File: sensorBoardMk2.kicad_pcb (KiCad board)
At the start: 2 copper layers, 42.3 x 63 mm, 45 parts, among them J1 S4B-PH-K-S__LF__SN_, J2 S4B-PH-K-S__LF__SN_, P1 TP, P2 TP, P3 TP, P4 TP, P5 TP, U1 SHT45, U2 BME280, U3 SGP40-D-R4

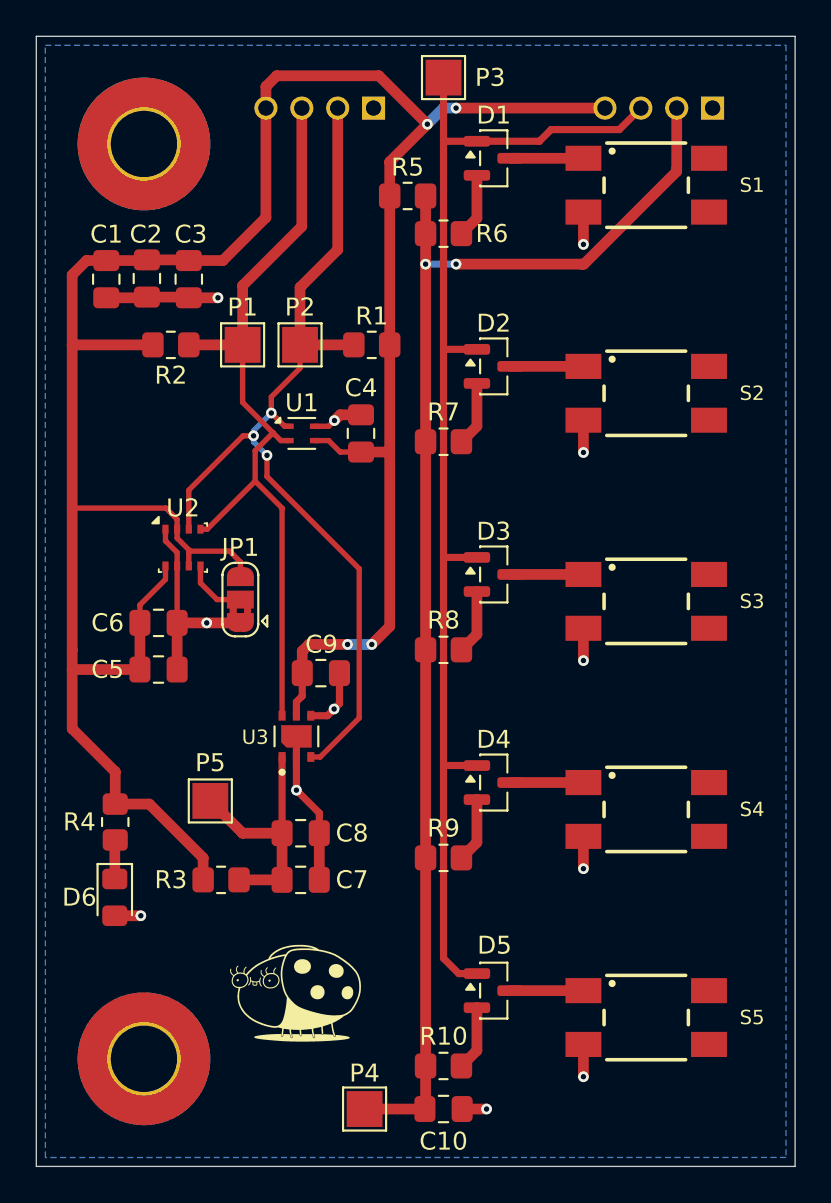
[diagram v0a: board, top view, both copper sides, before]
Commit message: Did some improvements based on feedback from lil brother
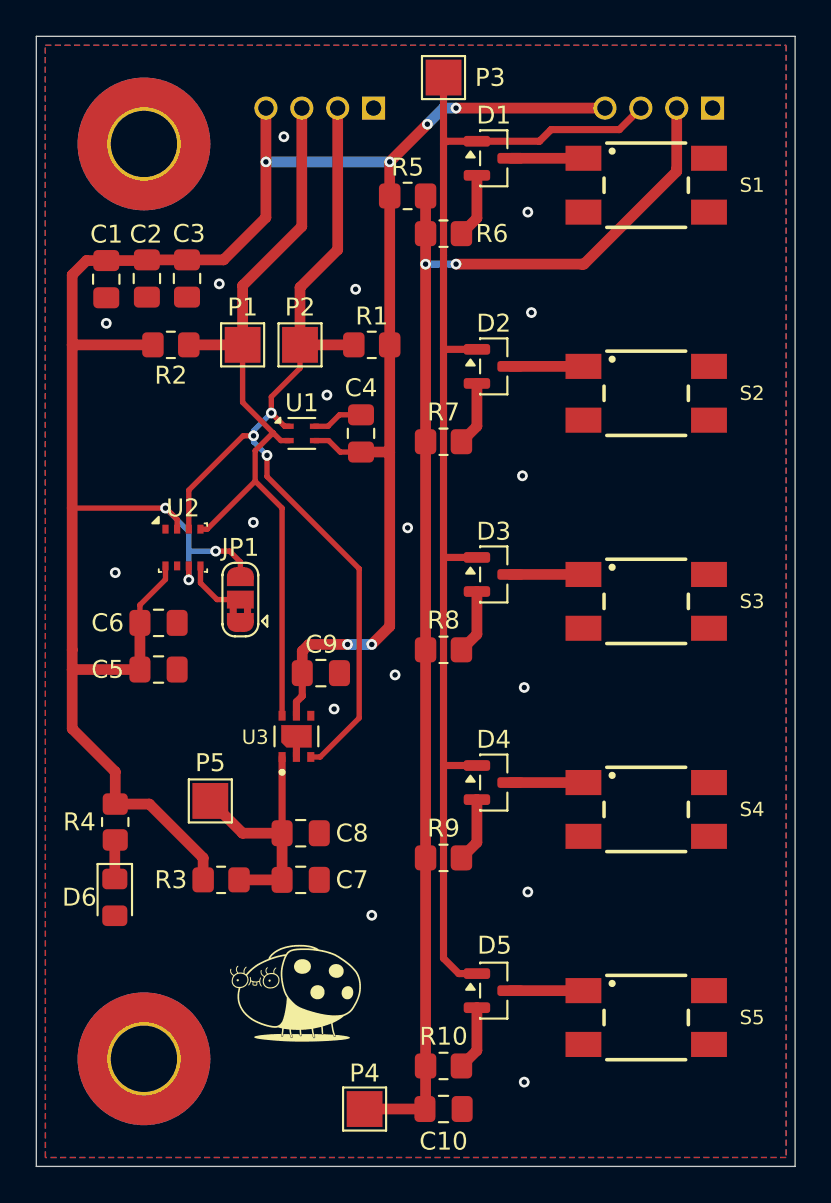
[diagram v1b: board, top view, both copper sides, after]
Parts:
- moved C3 0.11 mm to (49.1, 33.5)
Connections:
- MountingHoleBottom pad 1: (no net) -> GND
- MountingHoleTop pad 1: (no net) -> GND
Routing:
- net GND: track 44.7 -> 4.26 mm, vias 12 -> 17
- net +3.3V: track 148.2 -> 146.5 mm, vias 4 -> 9
- added copper zone on F.Cu, net GND
